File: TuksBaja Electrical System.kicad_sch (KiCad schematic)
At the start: 3 parts, among them U1 LM2596S-ADJ

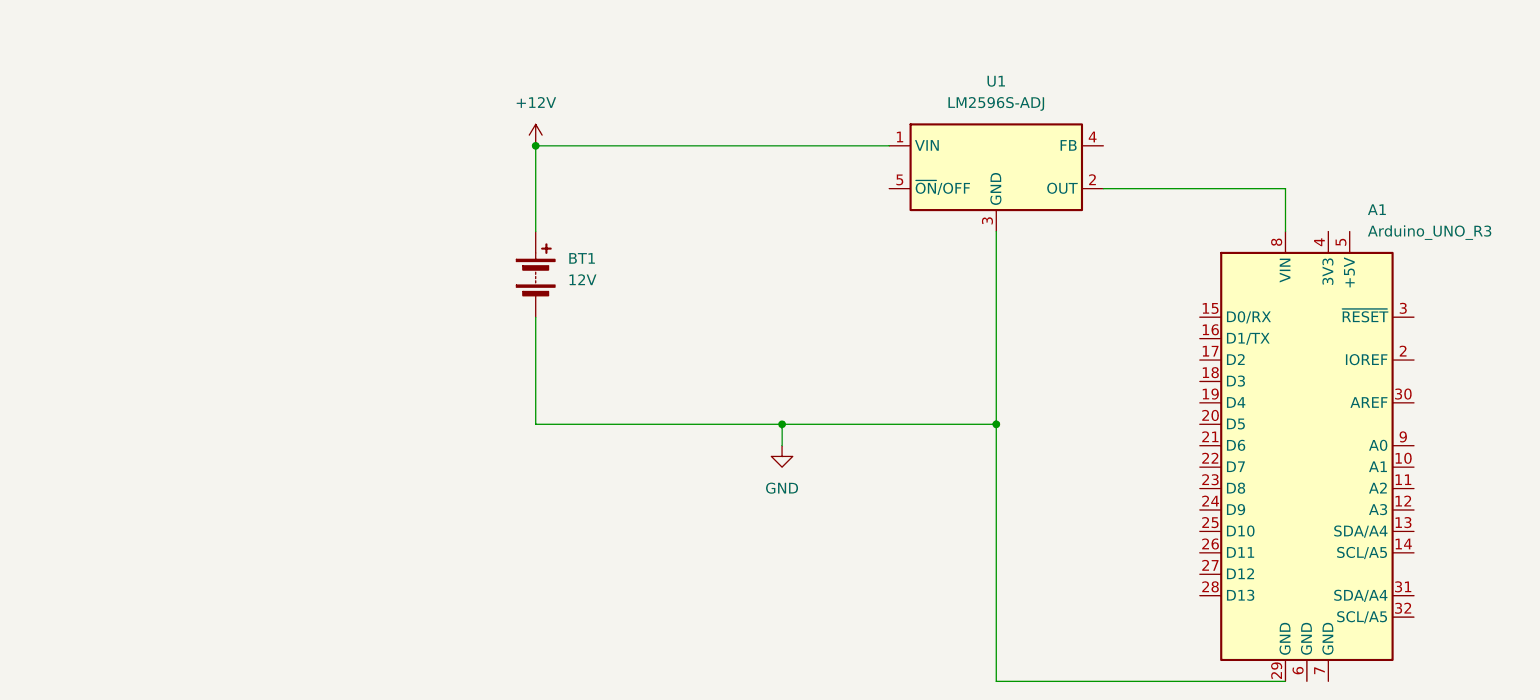
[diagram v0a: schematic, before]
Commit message: completed power supply
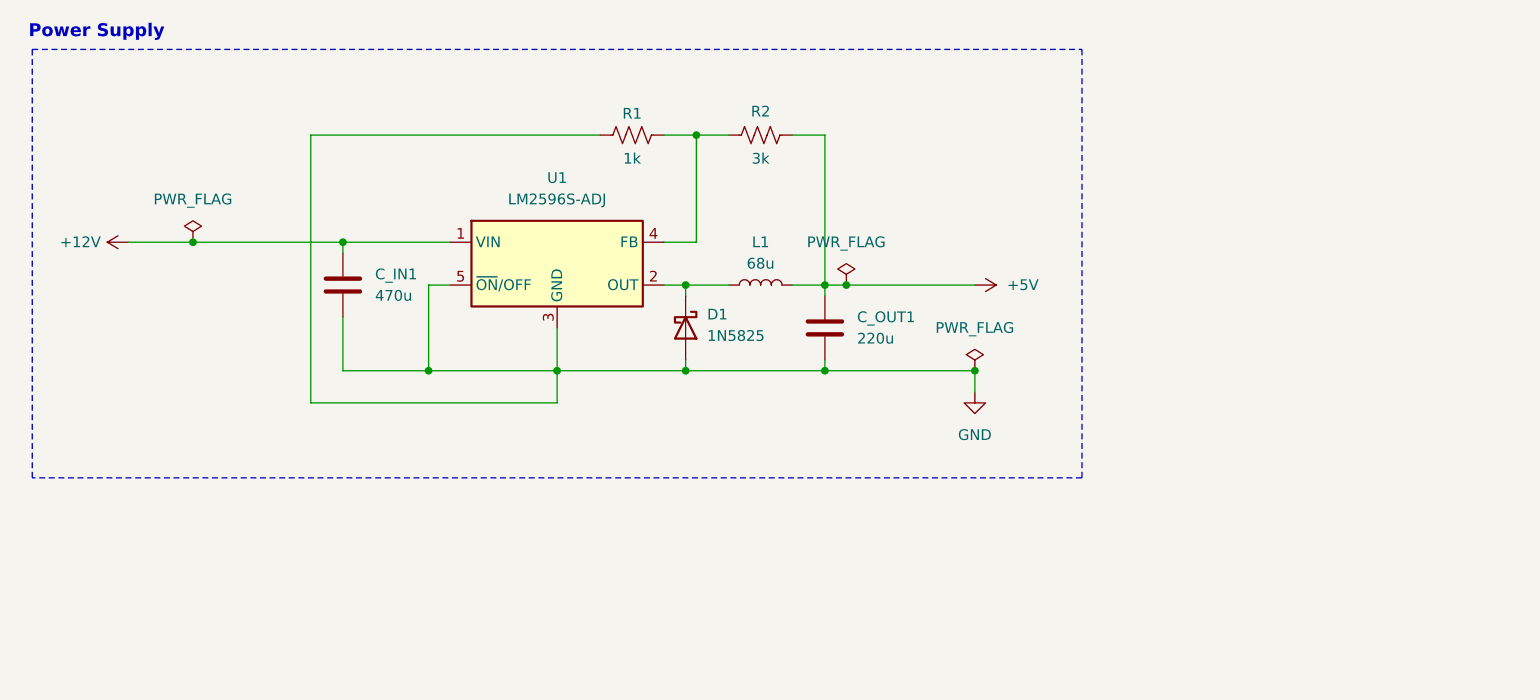
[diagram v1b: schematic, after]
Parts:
- removed A1: Arduino_UNO_R3, Module:Arduino_UNO_R3, symbol MCU_Module:Arduino_UNO_R3
- removed BT1: 12V, symbol Device:Battery
- added C_IN1: 470u, symbol Device:C
- added C_OUT1: 220u, symbol Device:C
- added D1: 1N5825, symbol Device:D_Schottky
- added L1: 68u, symbol Device:L
- added R1: 1k, symbol Device:R_US
- added R2: 3k, symbol Device:R_US
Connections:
- net +12V: now also C_IN1.1
- net GND: now also U1.5 (~{ON}/OFF), C_IN1.2, C_OUT1.2, D1.2 (A), R1.2
- net at U1.2 (OUT): now also D1.1 (K), L1.1
- net at U1.4 (FB): now also R1.1, R2.1
- new net +5V: C_OUT1.1, L1.2, R2.2
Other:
- note added: "Power Supply"
- company: (none) -> TuksBaja
- title: (none) -> Vehicle Electrical Schematic
